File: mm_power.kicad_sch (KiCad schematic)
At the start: 6 parts, among them J5 Conn_01x02, U4 LP5907MFX-3.3

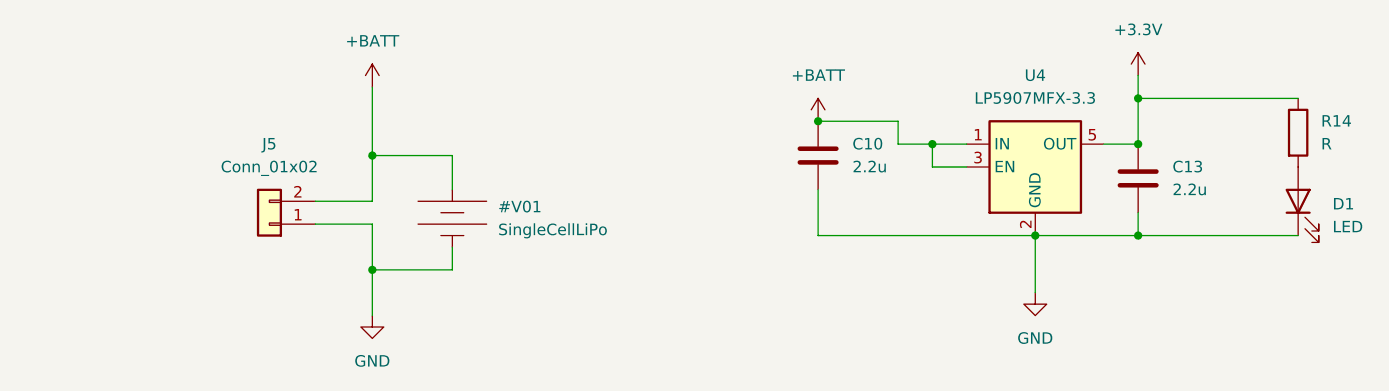
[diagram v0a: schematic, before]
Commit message: salimus
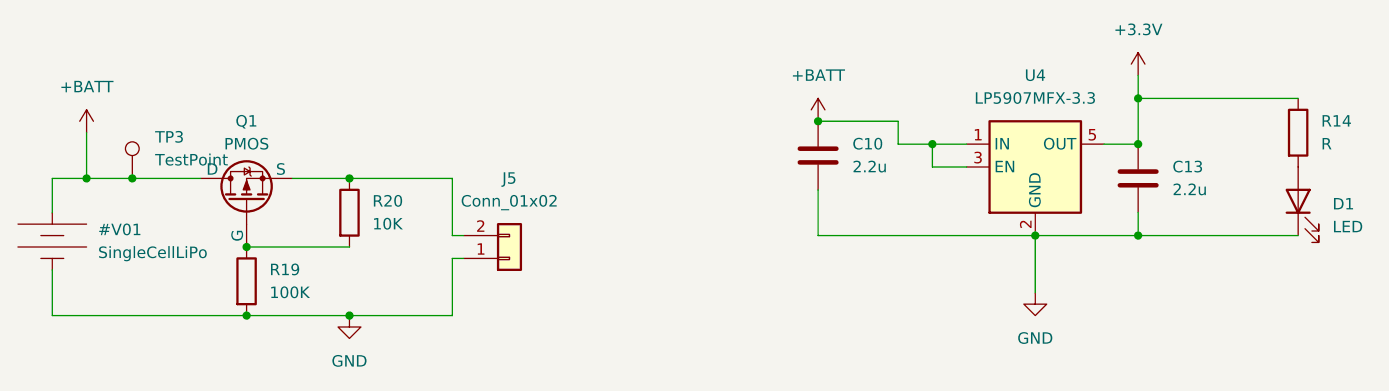
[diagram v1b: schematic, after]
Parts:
- added Q1: PMOS, Package_TO_SOT_SMD:SOT-23-3, symbol Simulation_SPICE:PMOS
- added R19: 100K, Resistor_SMD:R_0603_1608Metric, symbol Device:R
- added R20: 10K, Resistor_SMD:R_0603_1608Metric, symbol Device:R
- added TP3: TestPoint, TestPoint:TestPoint_Pad_D2.0mm, symbol Connector:TestPoint
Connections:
- net +BATT: now also Q1.1 (D), TP3.1; no longer J5.2 (Pin_2)
- net GND: now also R19.2
- new net: J5.2 (Pin_2), Q1.3 (S), R20.1
- new net: Q1.2 (G), R19.1, R20.2
